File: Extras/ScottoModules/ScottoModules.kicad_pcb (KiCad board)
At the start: 4 copper layers, 57.2 x 57.1 mm, 27 parts, among them J1 USB_C, SW1 SW_Push, U1 STM32F072CBT6, U3 XC6206, U4 USBLC6-2SC6

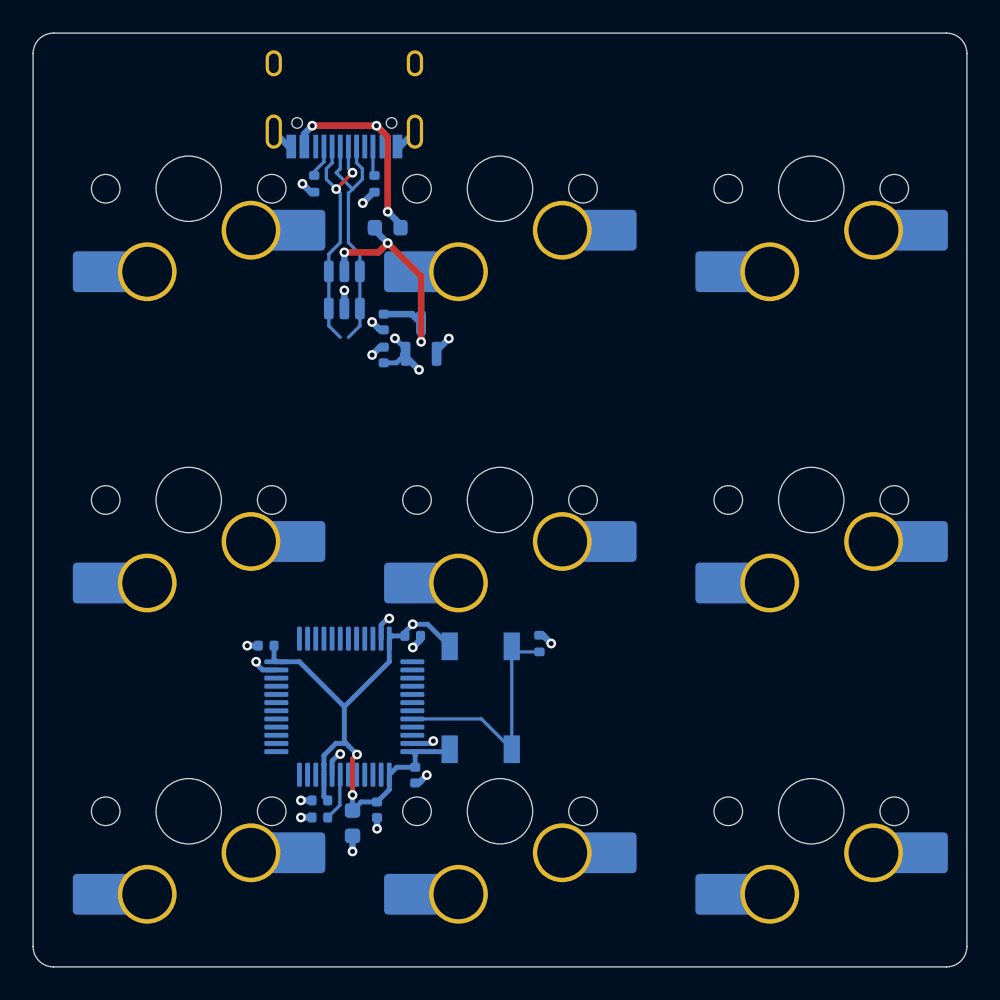
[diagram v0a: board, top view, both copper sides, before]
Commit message: Finalize modules
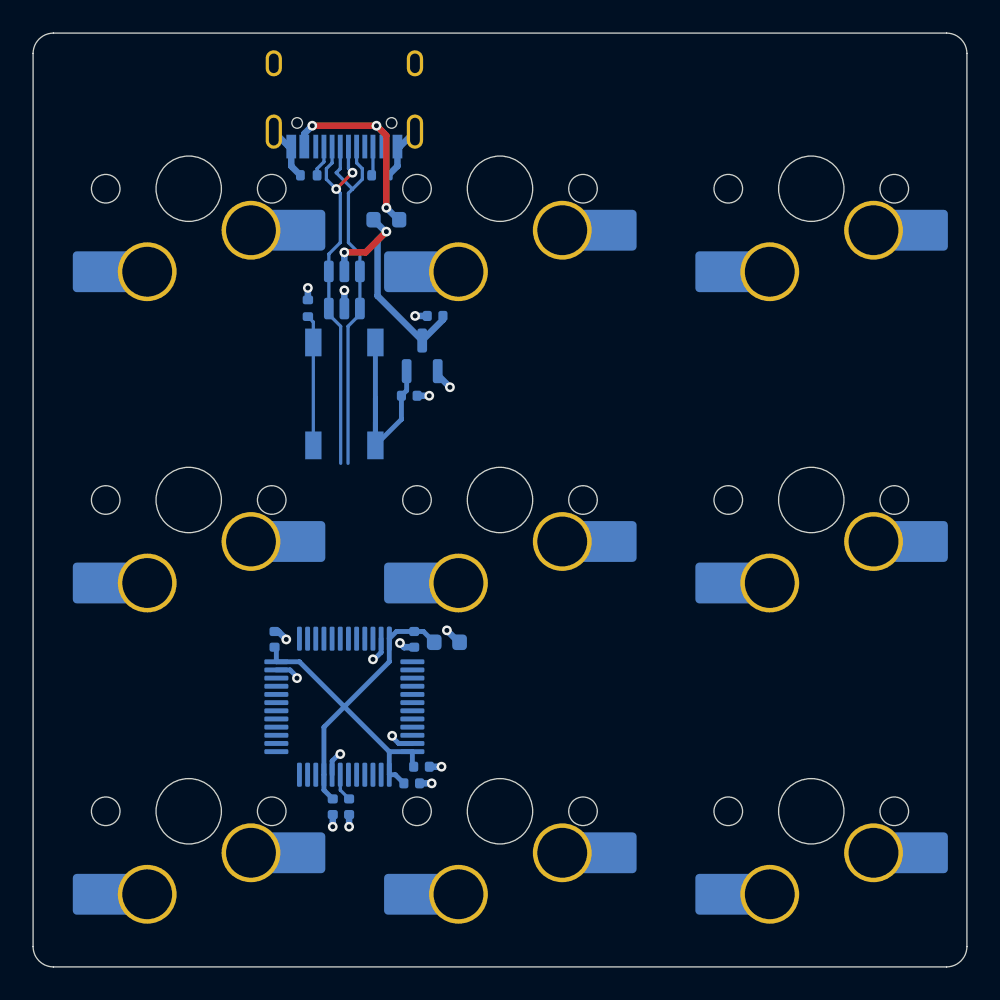
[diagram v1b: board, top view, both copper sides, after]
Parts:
- moved R1 24.9 mm to (428.0, 50.9)
- moved SW1 20.4 mm to (430.3, 56.1), turned to 90 degrees
- moved C6 12.5 mm to (436.5, 71.3), turned to 180 degrees
- moved C8 3.16 mm to (435.8, 51.3), turned to 180 degrees
- moved C9 2.94 mm to (434.2, 56.2), turned to 0 degrees
- moved C1 2.67 mm to (434.4, 80.0), turned to 180 degrees
- moved C7 1.91 mm to (430.6, 81.4), turned to -90 degrees
- moved U3 1.06 mm to (435.0, 53.8)
- moved C2 0.88 mm to (429.6, 81.4), turned to 90 degrees
- moved C5 0.64 mm to (435.0, 78.9), turned to 180 degrees
- moved C3 0.64 mm to (426.0, 71.1), turned to -90 degrees
- moved R3 0.62 mm to (432.4, 42.7), turned to 0 degrees
- moved R2 0.62 mm to (428.1, 42.7), turned to 180 degrees
- moved F1 0.50 mm to (432.8, 45.5)
- moved C4 0.23 mm to (434.5, 71.1), turned to 90 degrees
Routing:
- net D+: track 15.9 -> 23.6 mm
- net D-: track 16.0 -> 23.7 mm
- net BOOT0: track 15.0 -> 8.55 mm
- net +3.3V: track 40.8 -> 46.8 mm, vias 5 -> 0
- net GND: track 22.0 -> 23.5 mm, vias 18 -> 16
- net +5V: track 16.7 -> 15.4 mm, vias 3 -> 2
- net Net-(U1-NRST): track 2.94 -> 1.70 mm
- removed copper zone on In1.Cu, net GND
- removed copper zone on In2.Cu, net GND
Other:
- copper layers 4 -> 2
